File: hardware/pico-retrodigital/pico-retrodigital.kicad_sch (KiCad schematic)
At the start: 39 parts, among them J1 Conn_02x05_Top_Bottom, J2 HDMI_A, J3 Conn_01x03, J4 Conn_01x02_Pin, SW1 SW_Push, U1 74LVC2G17, U2 74LVC2G17, U3 SN74LVC8T245, U4 SN74LVC8T245, U5 74LVC2G17, U6 74LVC2G17, U7 RP2350B, Y1 ABM8-272-T3

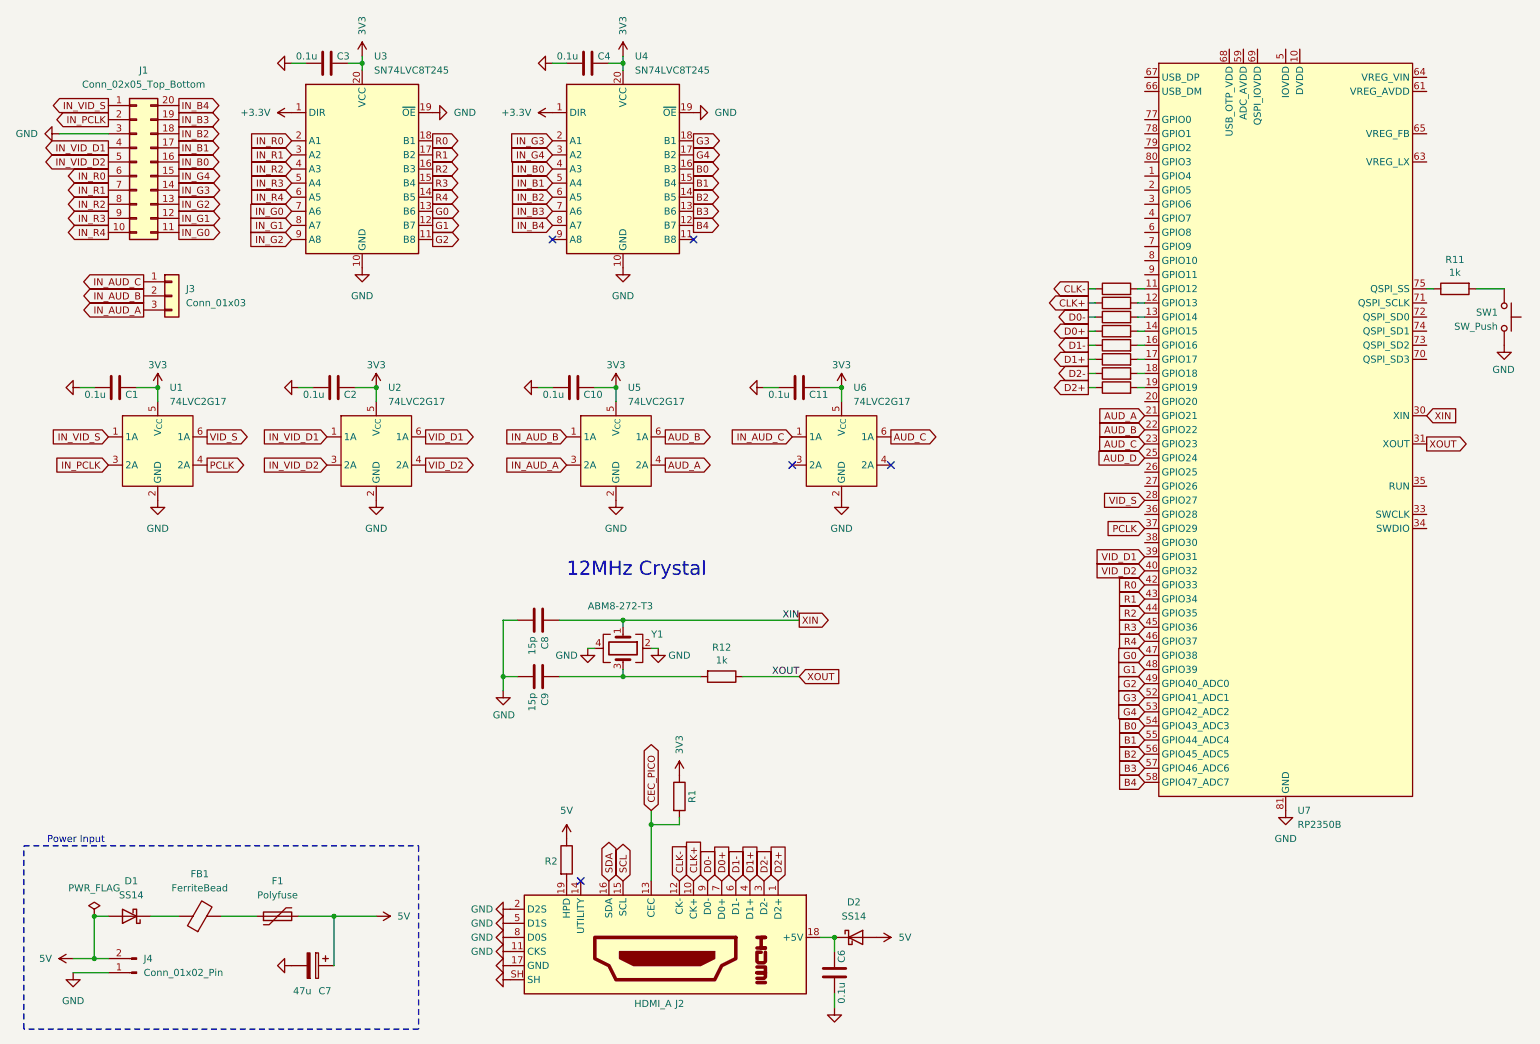
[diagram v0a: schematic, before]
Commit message: PCB update
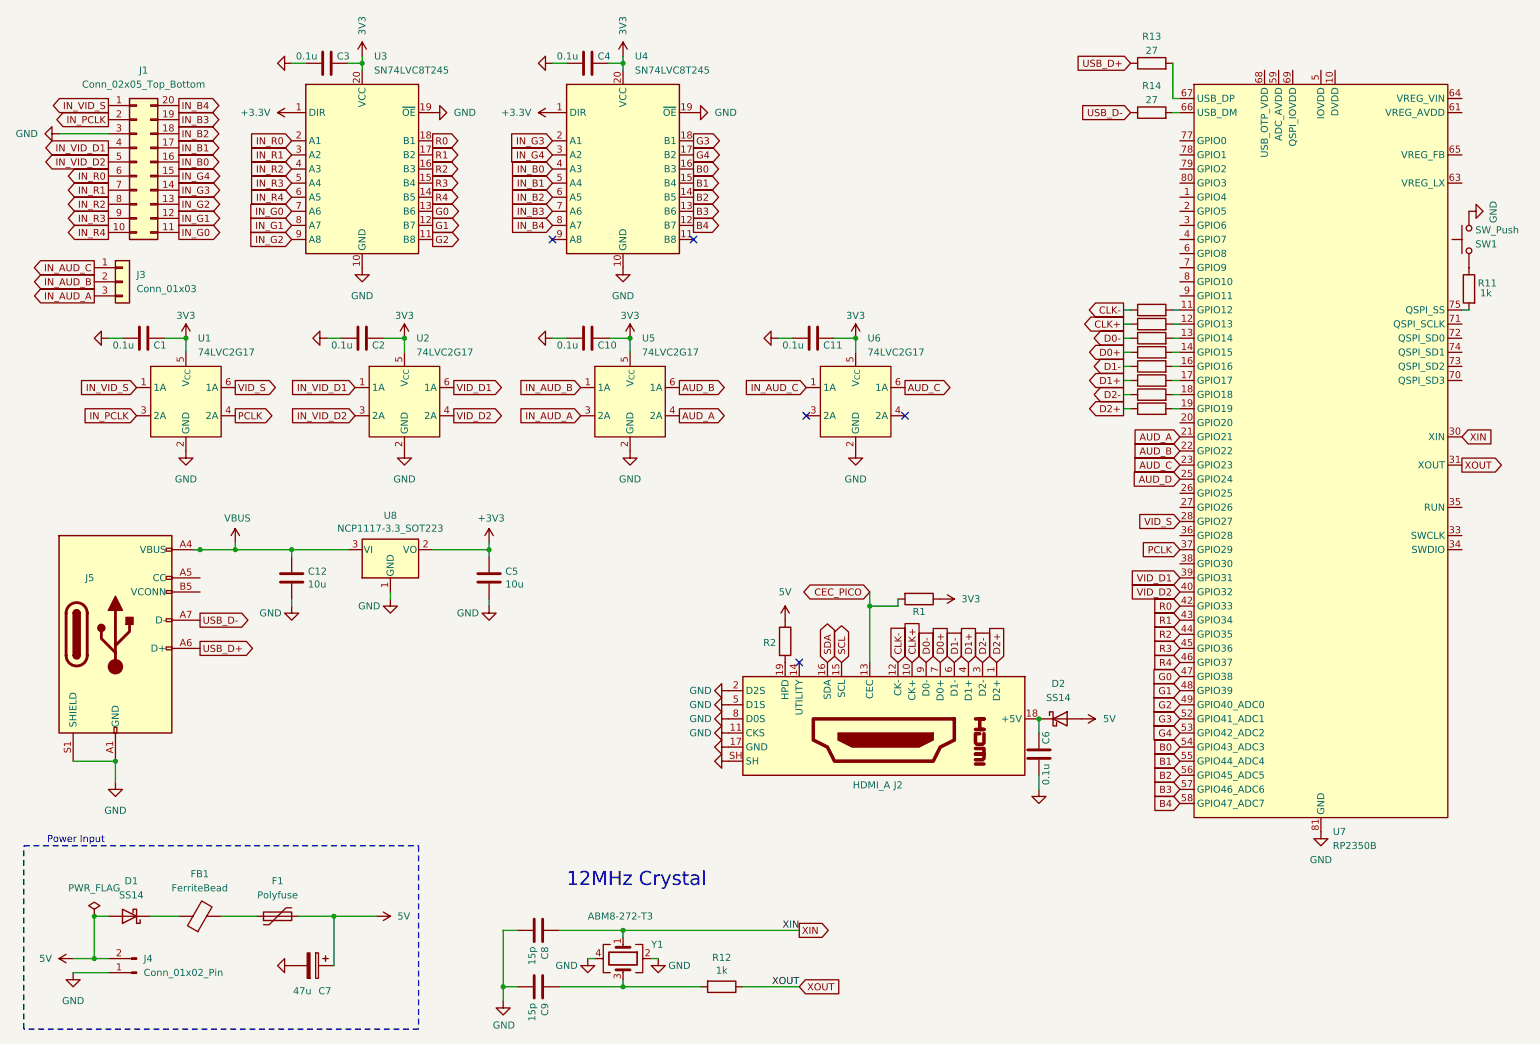
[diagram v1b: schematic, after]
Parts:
- added C12, C5: 10u, Capacitor_SMD:C_0805_2012Metric, symbol Device:C
- added J5: USB_C, Connector_USB:USB_Micro-B_Amphenol_10103594-0001LF_Horizontal, symbol Connector:USB_C_Plug_USB2.0
- added R13, R14: 27, Resistor_SMD:R_0402_1005Metric, symbol Device:R
- added U8: NCP1117-3.3_SOT223, Package_TO_SOT_SMD:SOT-223-3_TabPin2, symbol Regulator_Linear:NCP1117-3.3_SOT223
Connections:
- net GND: now also C12.2, C5.2, J5.A1 (GND), J5.A12 (GND), J5.B1 (GND), J5.B12 (GND), J5.S1 (SHIELD), U8.1 (GND)
- net at R11.1: now also SW1.2; no longer U7.75 (QSPI_SS)
- net at R11.2: now also U7.75 (QSPI_SS); no longer SW1.2
- net at U7.66 (USB_DM): now also R14.2
- net at U7.67 (USB_DP): now also R13.2
- new net +3V3: C5.1, U8.2 (VO)
- new net USB_D+: J5.A6 (D+), R13.1
- new net USB_D-: J5.A7 (D-), R14.1
- new net VBUS: C12.1, J5.A4 (VBUS), J5.A9 (VBUS), J5.B4 (VBUS), J5.B9 (VBUS), U8.3 (VI)
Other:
- moved on the sheet: C1, C10, C11, C2, C6, C8, C9, D2, J2, J3, R1, R11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
